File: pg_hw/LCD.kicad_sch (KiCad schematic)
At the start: 28 parts, among them J2 FPC_Touch, J3 FPC_Display, U10 ttp233, U11 ttp233, U8 ttp233, U9 TTP233

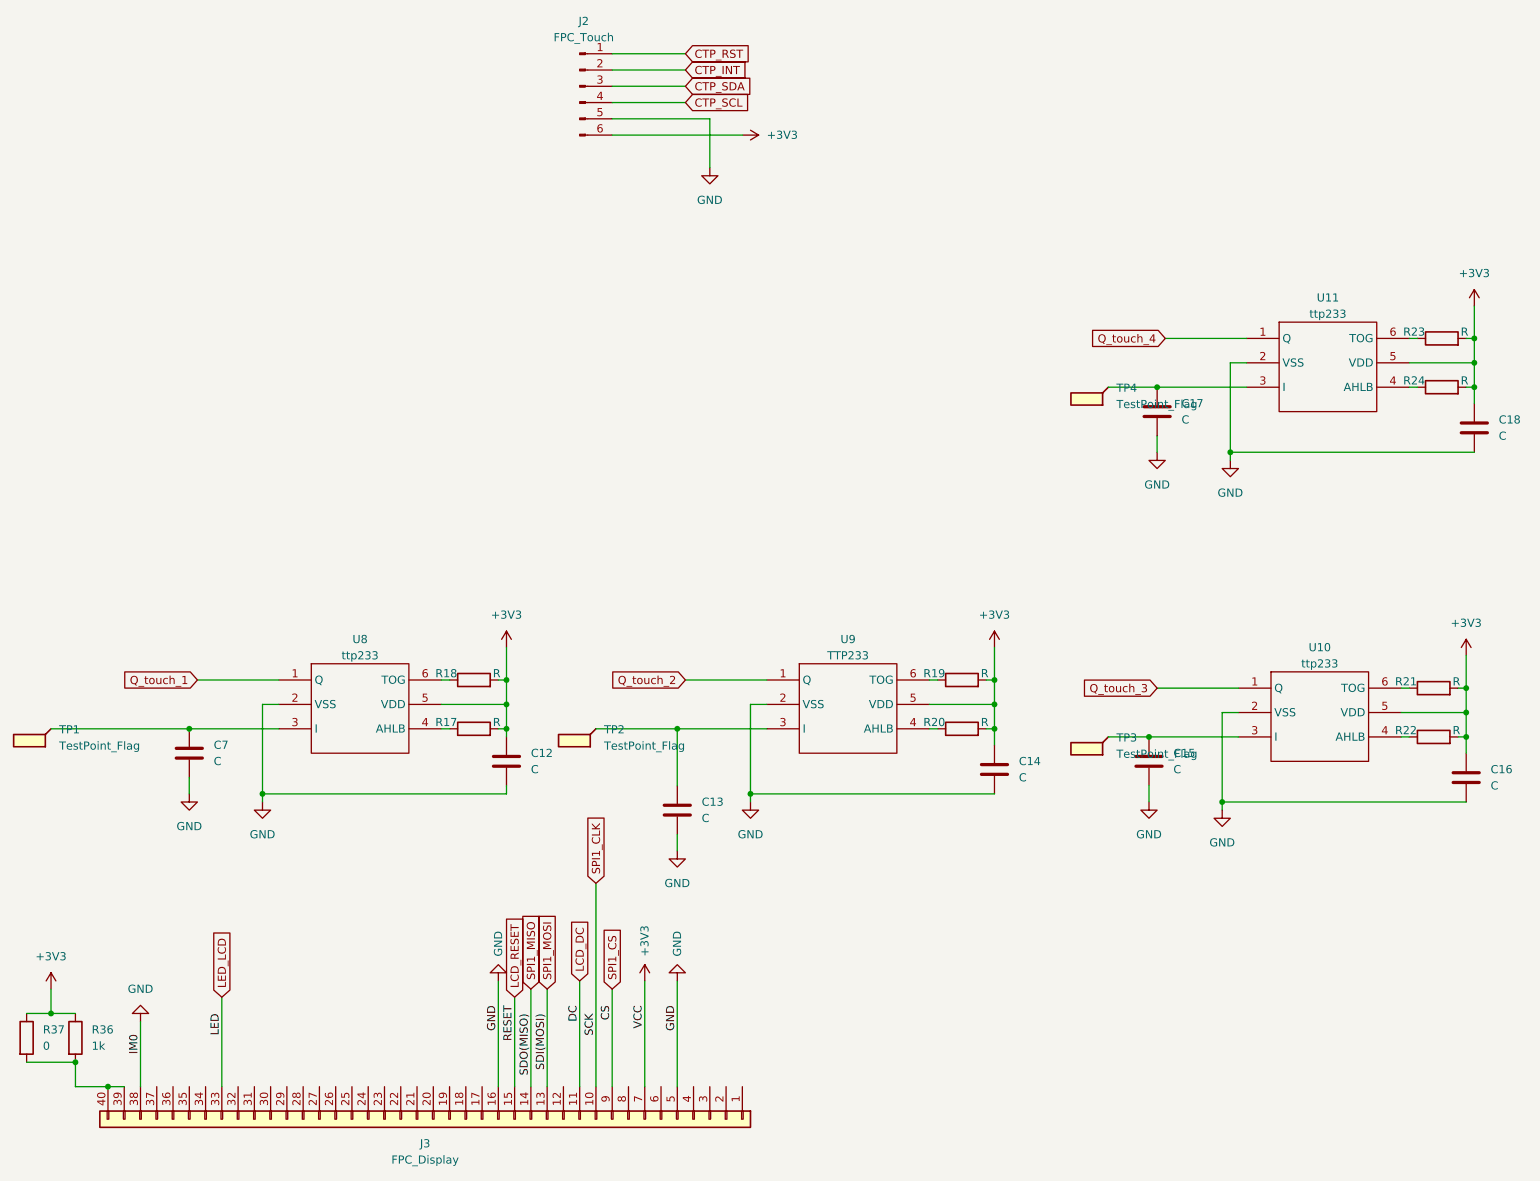
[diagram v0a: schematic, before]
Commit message: adad
dada
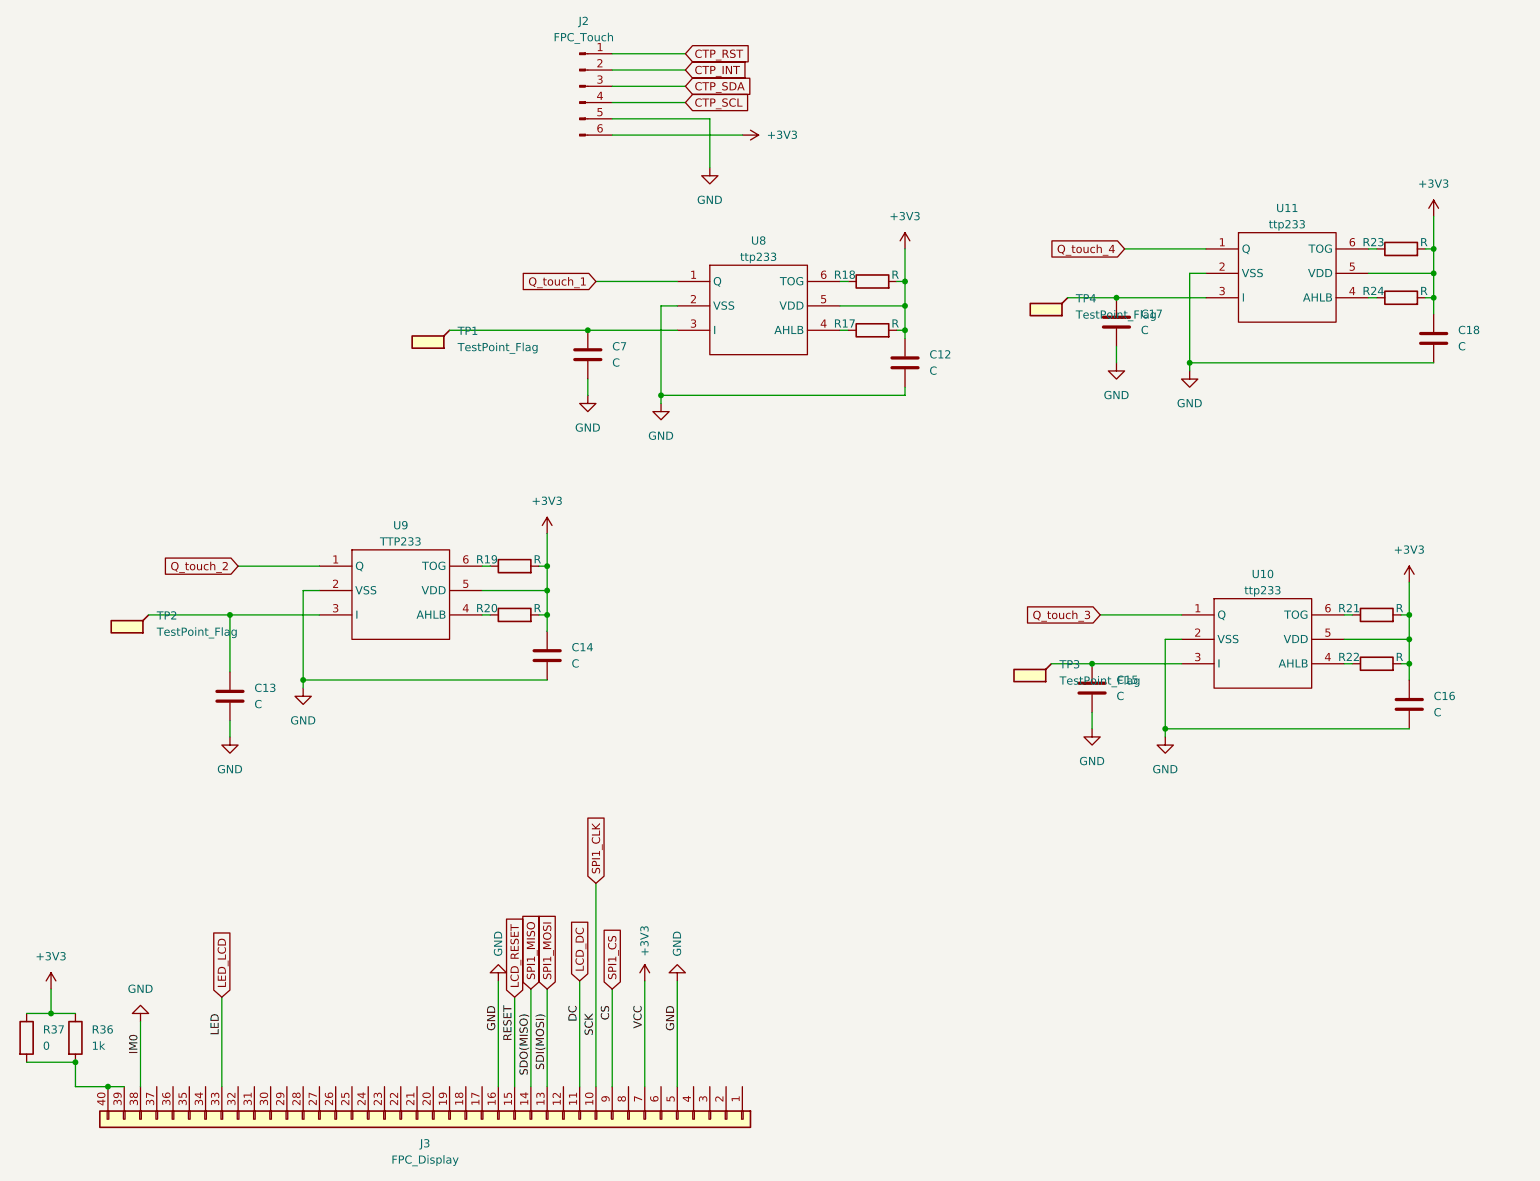
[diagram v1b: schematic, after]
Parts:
- C12, C13, C14, C15, C16, C17, C18, C7: footprint (none) -> Capacitor_SMD:C_0603_1608Metric
- R17, R18, R19, R20, R21, R22, R23, R24, R36, R37: footprint (none) -> Resistor_SMD:R_0402_1005Metric
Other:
- moved on the sheet: C12, C13, C14, C15, C16, C17, C18, C7, R17, R18, R19, R20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
